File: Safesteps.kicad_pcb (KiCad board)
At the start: 2 copper layers, 61 x 70.8 mm, 15 parts, among them J1 Conn_01x06_Pin, J2 Conn_01x05_Pin, SW1 SW_Push, U3 3.3 V, U4 ESP32-DEVKIT-V1

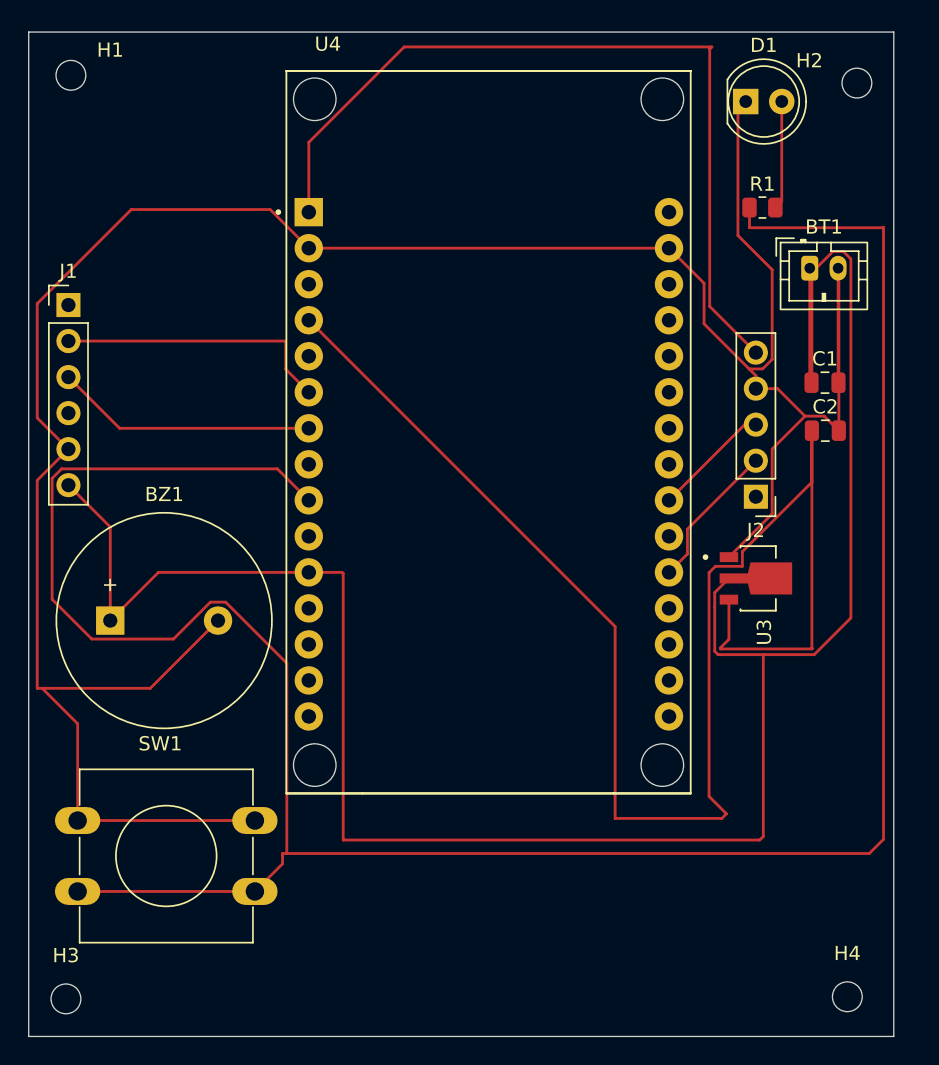
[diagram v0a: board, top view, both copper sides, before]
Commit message: Characteristics added
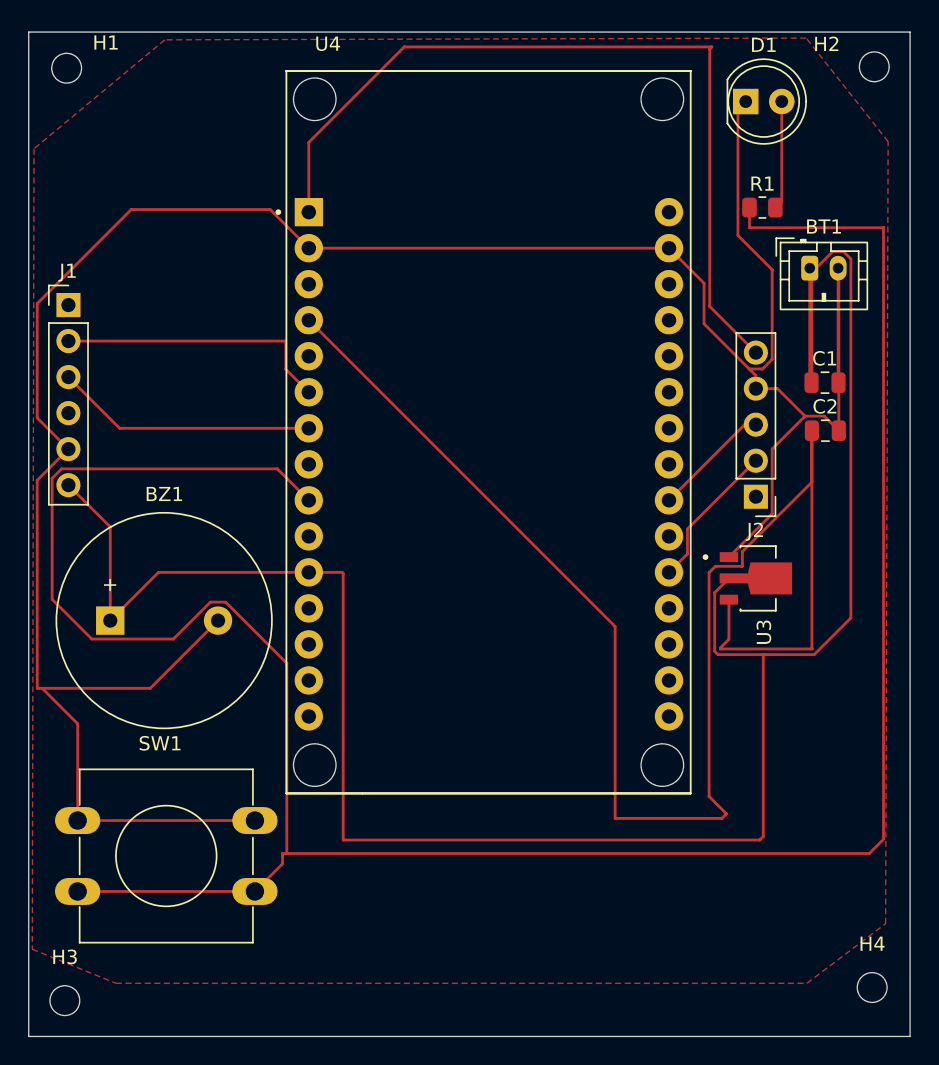
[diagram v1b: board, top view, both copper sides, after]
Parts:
- moved H4 1.87 mm to (146.3, 123.7)
- moved H2 1.68 mm to (146.5, 58.8)
- moved H1 0.58 mm to (89.5, 58.9)
- moved H3 0.15 mm to (89.4, 124.6)
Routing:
- added copper zone on F.Cu, net GND
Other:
- board size 61 x 70.8 mm -> 62.2 x 70.8 mm
